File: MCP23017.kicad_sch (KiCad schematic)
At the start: 29 parts, among them J10 Conn_PH_01x10, J2 Carte_Relais, J3 Conn_03x08_Odd_Even, J5 Conn_03x08_Odd_Even, J8 Conn_PH_01x10, J9 Conn_03x08_Odd_Even, U2 MCP23017, U3 MCP23017, U4 ULN2803ADWR

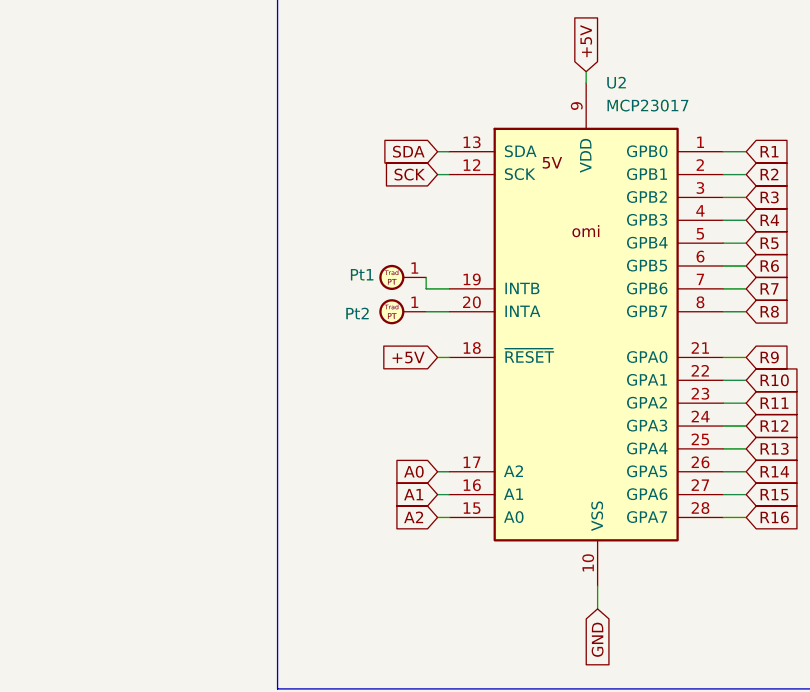
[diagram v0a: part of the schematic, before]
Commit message: 26/06/2025  8:54 Signed-off-by: TEST-BANC <TEST-BANC@DOMOMICRON.LOCAL>
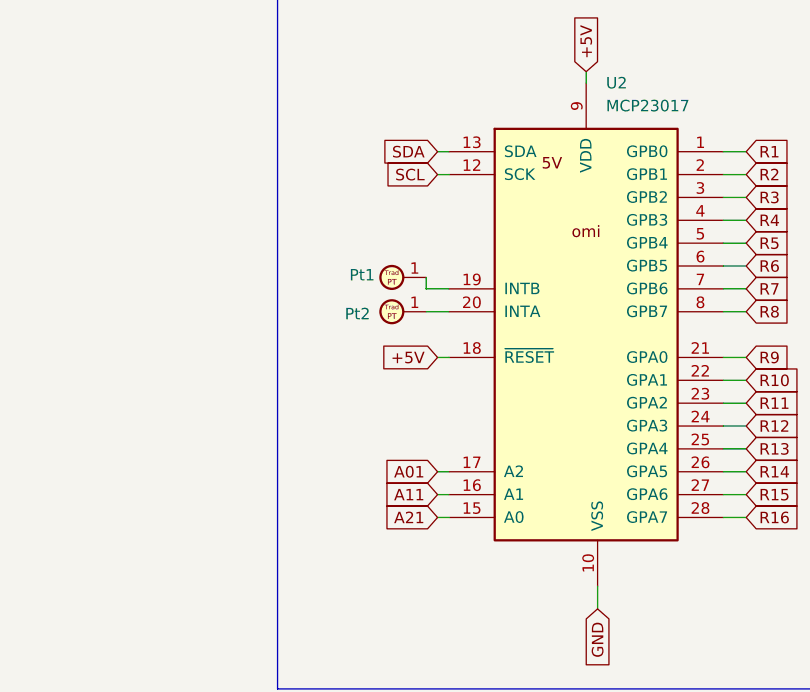
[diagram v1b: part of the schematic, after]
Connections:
- net A0 is gone; now on net A01: U2.17 (A2)
- net A1 is gone; now on net A11: U2.16 (A1)
- net A2 is gone; now on net A21: U2.15 (A0)
- net SCK: no longer U2.12 (SCK)
- new net SCL: U2.12 (SCK)
